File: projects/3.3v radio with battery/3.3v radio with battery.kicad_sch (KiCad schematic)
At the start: 15 parts, among them J1 USB_B

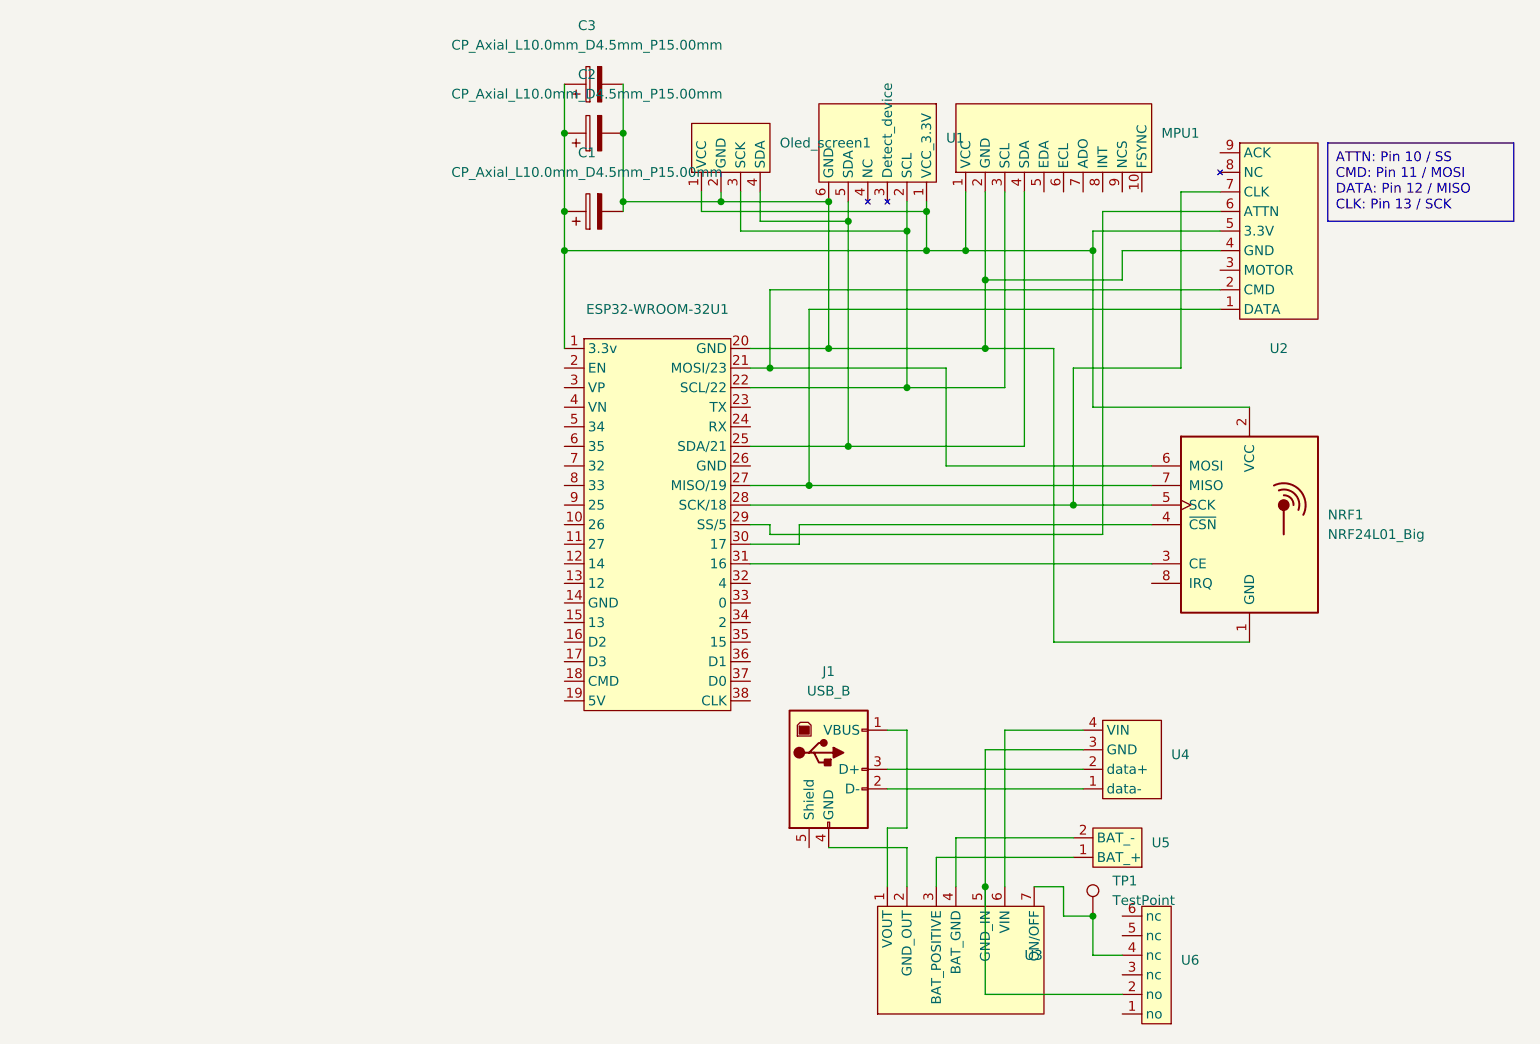
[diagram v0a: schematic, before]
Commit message: only multi remote left
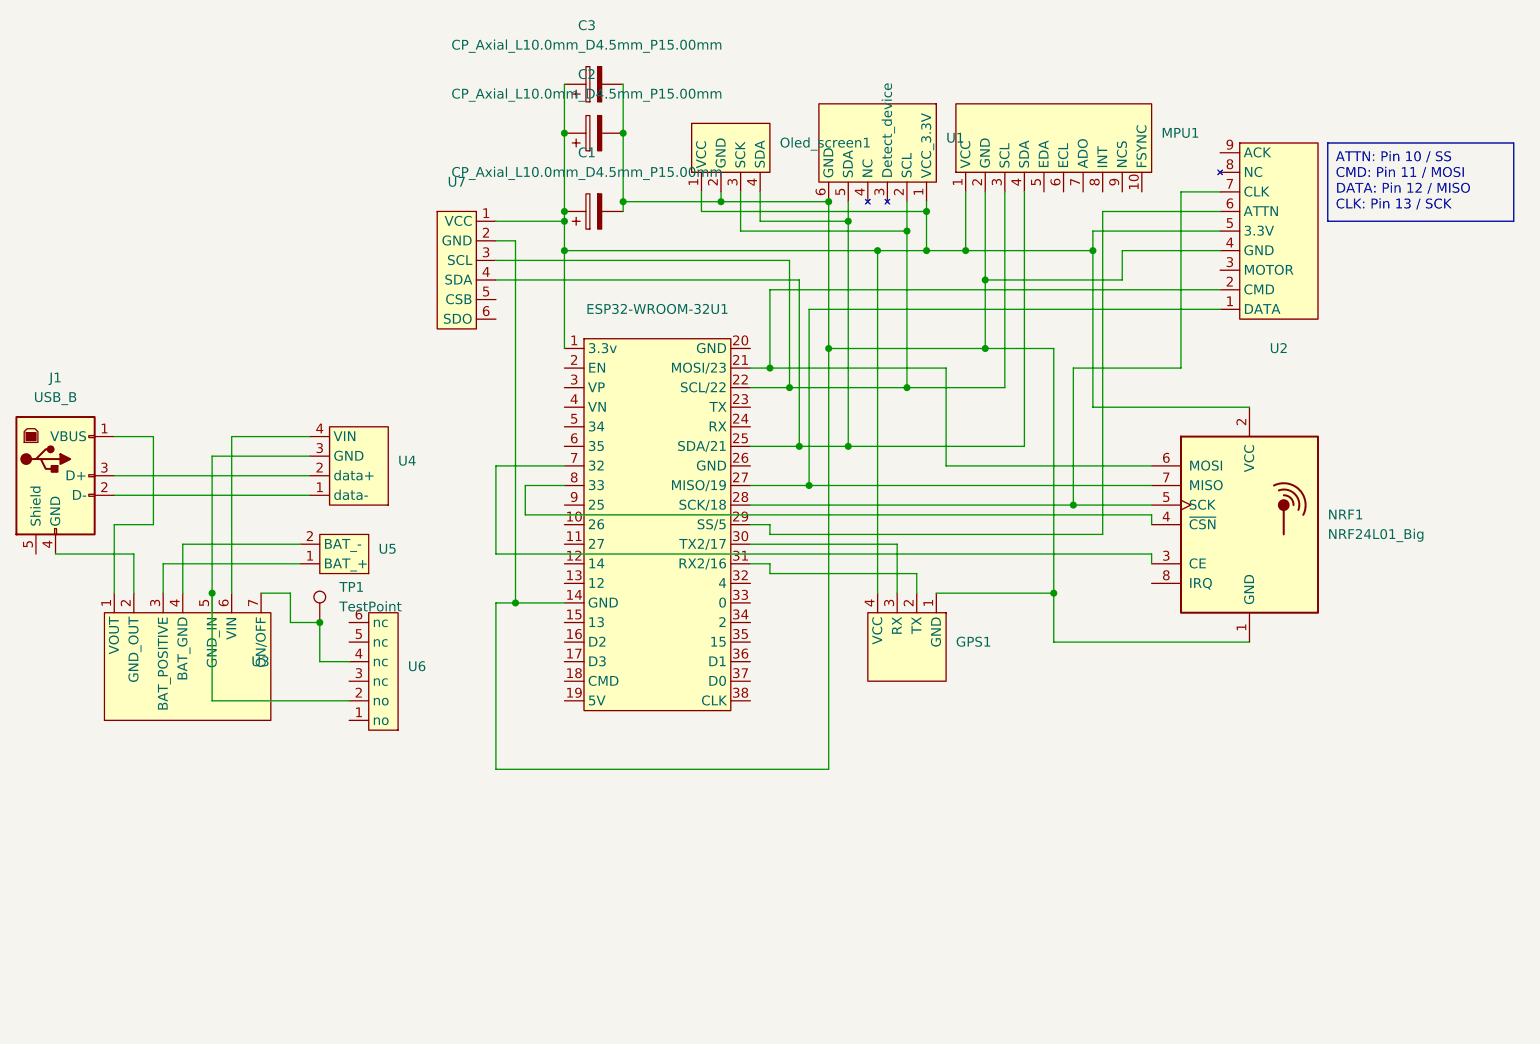
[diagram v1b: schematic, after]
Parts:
- added GPS1: ~, Footprints_cez:GY-NEO6MV2_flipped, symbol Symbols_cez:GY-NEO6MV2
- added U7: ~, Footprints_cez:BME280, symbol Symbols_cez:BME280_3.3V
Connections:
- net at C1.2, C2.2, C3.2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: now also ESP32-WROOM-32U1.14 (GND), GPS1.1 (GND), U7.2 (GND); no longer ESP32-WROOM-32U1.20 (GND)
- net at C1.1, C2.1, C3.1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: now also GPS1.4 (VCC), U7.1 (VCC)
- net at NRF1.3 (CE): now also ESP32-WROOM-32U1.7 (32); no longer ESP32-WROOM-32U1.31 (16)
- net at NRF1.4 (~{CSN}): now also ESP32-WROOM-32U1.8 (33); no longer ESP32-WROOM-32U1.30 (17)
- net at ESP32-WROOM-32U1.22 (SCL/22), MPU1.3 (SCL), Oled_screen1.3 (SCK)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: now also U7.3 (SCL)
- net at ESP32-WROOM-32U1.25 (SDA/21), MPU1.4 (SDA), Oled_screen1.4 (SDA)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: now also U7.4 (SDA)
- new net: ESP32-WROOM-32U1.31 (RX2/16), GPS1.2 (TX)
- new net: ESP32-WROOM-32U1.30 (TX2/17), GPS1.3 (RX)
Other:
- moved on the sheet: J1, TP1, U3, U4, U5, U6
